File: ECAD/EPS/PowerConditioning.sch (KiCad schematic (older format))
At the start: 87 parts, among them Q10 SIR167DP, Q11 SIR167DP, Q12 2N7002, Q13 IRF7458, Q14 2N7002, Q15 2N7002, Q16 2N7002, Q17 IRF7458, Q18 IRF7458, Q19 2N7002, Q20 2N7002, Q7 IRF7458, Q8 2N7002, Q9 IRF7458, SW3 INHIBIT 3, U26 LM358, U27 ADR4530, U28 MAX1626, U29 MAX1626, U30 LM1117-3.3, U31 MAX4373F, U32 MAX4373F, U33 MAX4373F

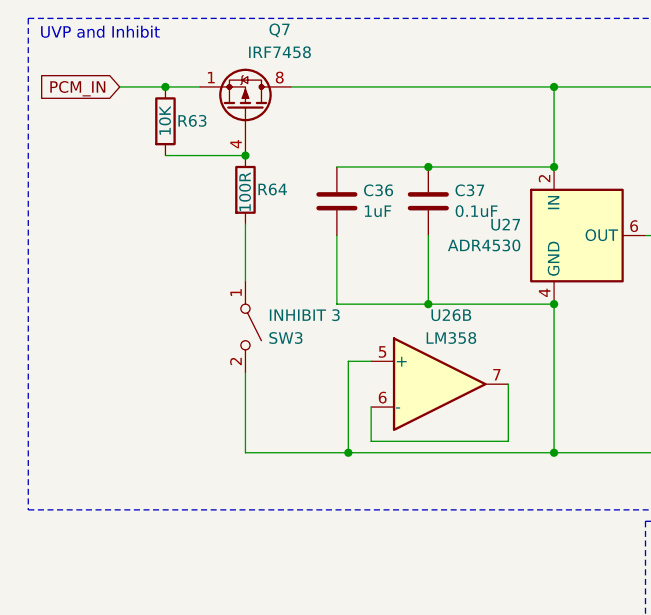
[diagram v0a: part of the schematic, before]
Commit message: inhibit resistor values, among other things
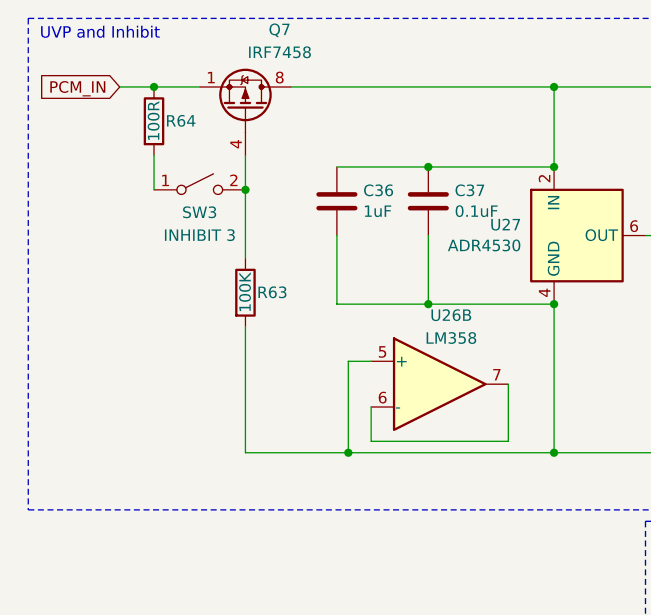
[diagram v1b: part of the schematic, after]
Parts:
- R63: value 10K -> 100K
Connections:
- net GND: now also R63.2; no longer SW3.2 (B)
- net PCM_IN: now also R64.1; no longer R63.1
- new net: Q7.4 (G), R63.1, SW3.2 (B)
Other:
- moved on the sheet: R63, R64, SW3
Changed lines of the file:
@@
 	0    1    1    0
 $EndComp
-Connection ~ 1450 1100
 $Comp
 L Device:R R?
 U 1 1 61ECA4CA
-P 1450 1250
+P 1050 950
 AR Path="/61BEC565/61ECA4CA" Ref="R?"  Part="1"
 AR Path="/61C9425D/61ECA4CA" Ref="R64"  Part="1"
-F 0 "R64" H 1500 1250 50  0000 L CNN
-F 1 "100R" V 1450 1150 50  0000 L CNN
-F 2 "Resistor_SMD:R_0805_2012Metric" V 1380 1250 50  0001 C CNN
-F 3 "~" H 1450 1250 50  0001 C CNN
-	1    1450 1250
+F 0 "R64" H 1100 950 50  0000 L CNN
+F 1 "100R" V 1050 950 50  0000 C CNN
+F 2 "Resistor_SMD:R_0805_2012Metric" V 980 950 50  0001 C CNN
+F 3 "~" H 1050 950 50  0001 C CNN
+	1    1050 950
 	1    0    0    -1
 $EndComp
 $Comp
-L Switch:SW_SPST SW?
-U 1 1 61ECA4D0
-P 1450 1850
-AR Path="/61BEC565/61ECA4D0" Ref="SW?"  Part="1"
-AR Path="/61C9425D/61ECA4D0" Ref="SW3"  Part="1"
-F 0 "SW3" V 1500 1950 50  0000 L CNN
-F 1 "INHIBIT 3" V 1400 1950 50  0000 L CNN
-F 2 "Connector_Hirose:Hirose_DF13-02P-1.25DSA_1x02_P1.25mm_Vertical" H 1450 1850 50  0001 C CNN
-F 3 "~" H 1450 1850 50  0001 C CNN
-	1    1450 1850
-	0    1    1    0
-$EndComp
-Wire Wire Line
-	1100 1100 1450 1100
-Wire Wire Line
-	1250 800  1100 800
-$Comp
 L Device:R R?
 U 1 1 61ECA4D8
-P 1100 950
+P 1450 1700
 AR Path="/61BEC565/61ECA4D8" Ref="R?"  Part="1"
 AR Path="/61C9425D/61ECA4D8" Ref="R63"  Part="1"
-F 0 "R63" H 1150 950 50  0000 L CNN
-F 1 "10K" V 1100 950 50  0000 C CNN
-F 2 "Resistor_SMD:R_0805_2012Metric" V 1030 950 50  0001 C CNN
-F 3 "~" H 1100 950 50  0001 C CNN
-	1    1100 950
+F 0 "R63" H 1500 1700 50  0000 L CNN
+F 1 "100K" V 1450 1700 50  0000 C CNN
+F 2 "Resistor_SMD:R_0805_2012Metric" V 1380 1700 50  0001 C CNN
+F 3 "~" H 1450 1700 50  0001 C CNN
+	1    1450 1700
 	1    0    0    -1
 $EndComp
@@
 $EndComp
 Wire Wire Line
-	900  800  1100 800
-Connection ~ 1100 800
-Wire Wire Line
-	1450 1400 1450 1650
-Wire Wire Line
 	1650 800  2800 800
 Connection ~ 2800 800
-Wire Wire Line
-	1450 2050 1450 2400
 Wire Wire Line
 	1450 2400 1900 2400
@@
 Wire Notes Line
 	500  500  5500 500
+$Comp
+L Switch:SW_SPST SW?
+U 1 1 61ECA4D0
+P 1250 1250
+AR Path="/61BEC565/61ECA4D0" Ref="SW?"  Part="1"
+AR Path="/61C9425D/61ECA4D0" Ref="SW3"  Part="1"
+F 0 "SW3" H 1250 1150 50  0000 C CNN
+F 1 "INHIBIT 3" H 1250 1050 50  0000 C CNN
+F 2 "Connector_Hirose:Hirose_DF13-02P-1.25DSA_1x02_P1.25mm_Vertical" H 1250 1250 50  0001 C CNN
+F 3 "~" H 1250 1250 50  0001 C CNN
+	1    1250 1250
+	1    0    0    -1
+$EndComp
+Wire Wire Line
+	900  800  1050 800
+Connection ~ 1050 800
+Wire Wire Line
+	1050 800  1250 800
+Wire Wire Line
+	1450 1550 1450 1250
+Connection ~ 1450 1250
+Wire Wire Line
+	1450 1250 1450 1100
+Wire Wire Line
+	1050 1100 1050 1250
+Wire Wire Line
+	1450 1850 1450 2400
 $EndSCHEMATC
